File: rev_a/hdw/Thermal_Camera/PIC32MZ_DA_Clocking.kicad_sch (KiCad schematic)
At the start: 17 parts, among them U1101 74LVC1G97, X1101 ASE-8.000MHz, X1102 ECS-327KE

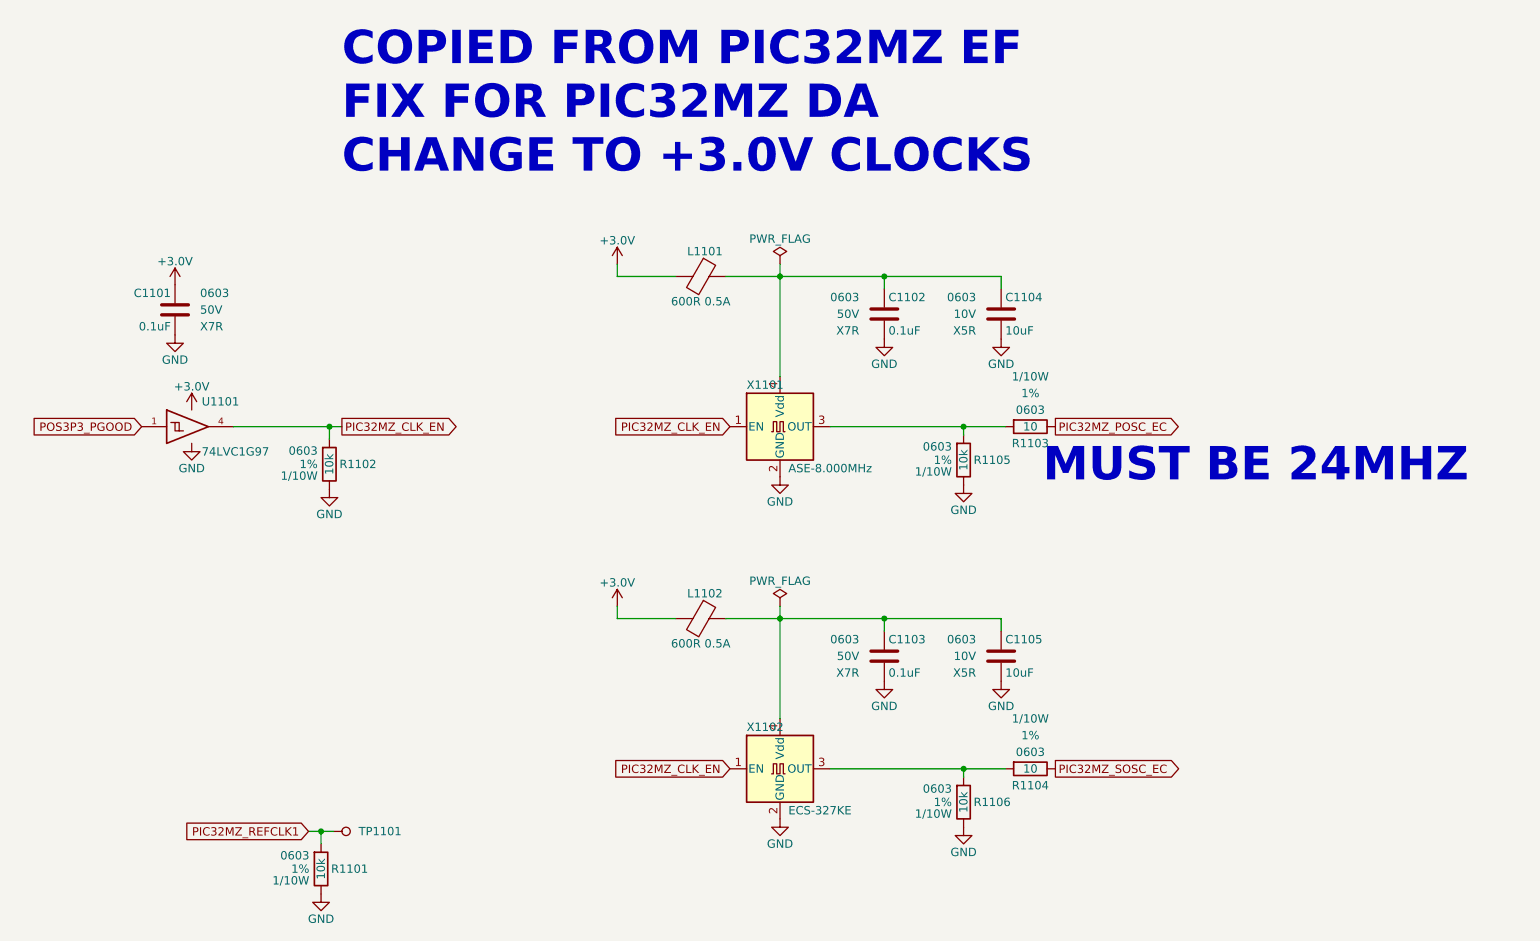
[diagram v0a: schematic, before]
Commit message: added PIC32 bypass, SD card load switch, other random junk
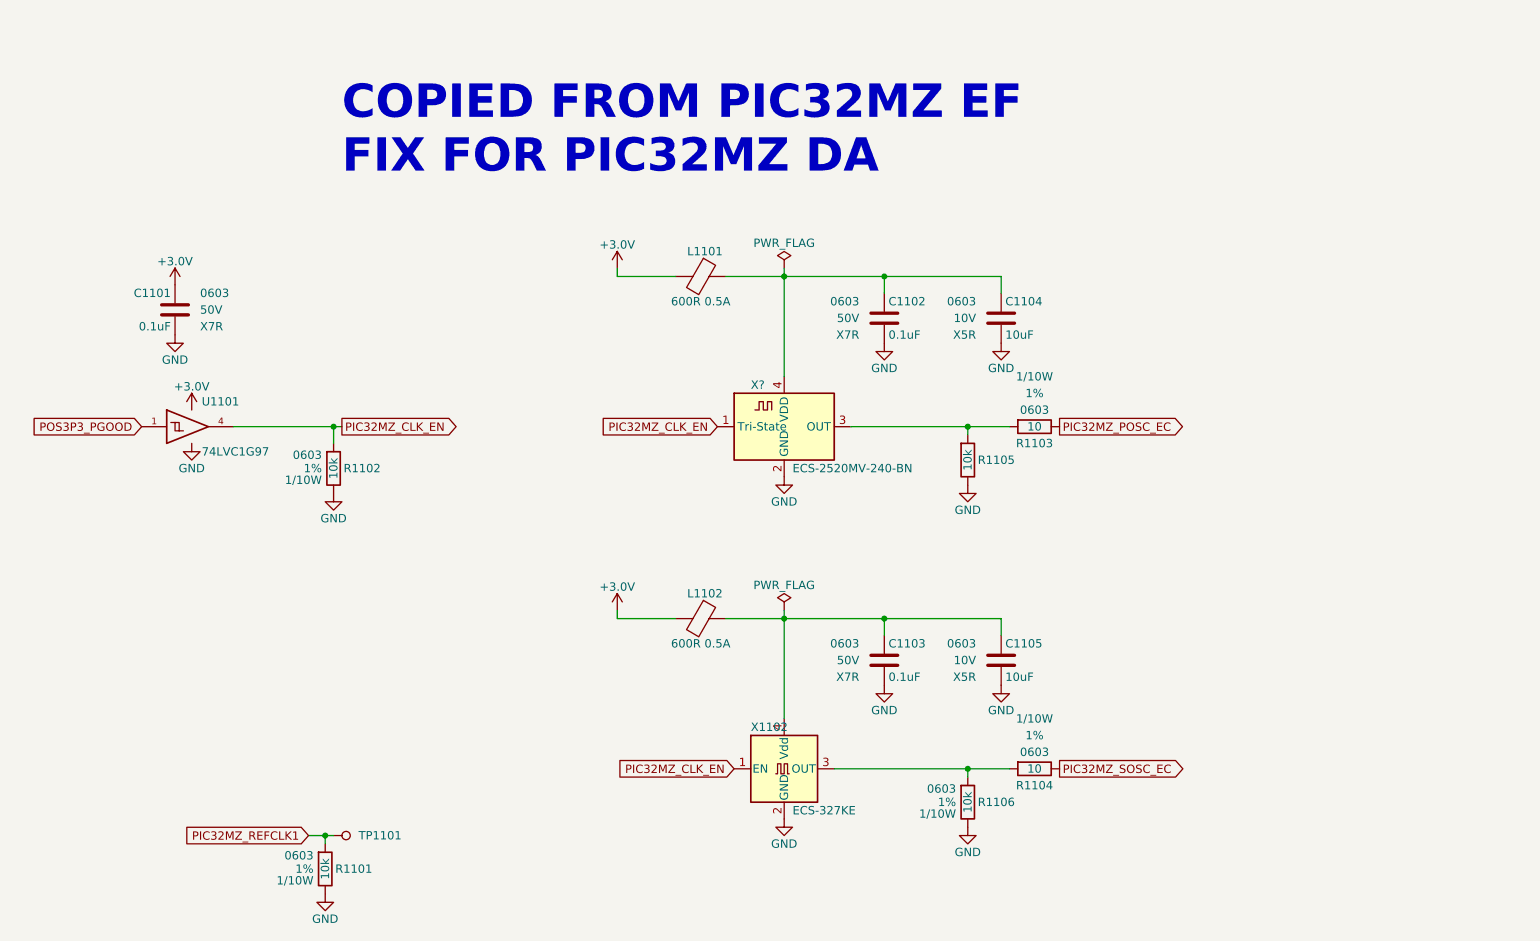
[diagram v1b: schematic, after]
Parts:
- removed X1101: ASE-8.000MHz, Oscillator:Oscillator_SMD_Abracon_ASE-4Pin_3.2x2.5mm, symbol Oscillator:ASE-xxxMHz
- added X?: ECS-2520MV-240-BN, Oscillator:Oscillator_SMD_ECS_2520MV-xxx-xx-4Pin_2.5x2.0mm, symbol Oscillator:ECS-2520MV-xxx-xx
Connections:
- net GND: now also X?.2 (GND)
- net PIC32MZ_CLK_EN: now also X?.1 (Tri-State)
- net at R1103.1, R1105.1: now also X?.3 (OUT)
- net at C1102.1, C1104.1, L1101.1: now also X?.4 (VDD)
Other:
- note added: "COPIED FROM PIC32MZ EF FIX FOR PIC32MZ DA"
- note removed: "COPIED FROM PIC32MZ EF FIX FOR PIC32MZ DA CHANGE TO +3.0V CLOCKS"
- note removed: "MUST BE 24MHZ"
- moved on the sheet: C1102, C1103, C1104, C1105, R1101, R1102, R1103, R1104, R1105, R1106, TP1101, X1102
